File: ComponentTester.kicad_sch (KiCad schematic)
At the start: 15 parts, among them J11 Conn_01x02, J2 Conn_01x03, J3 Conn_01x02, U2 OPA188xxD

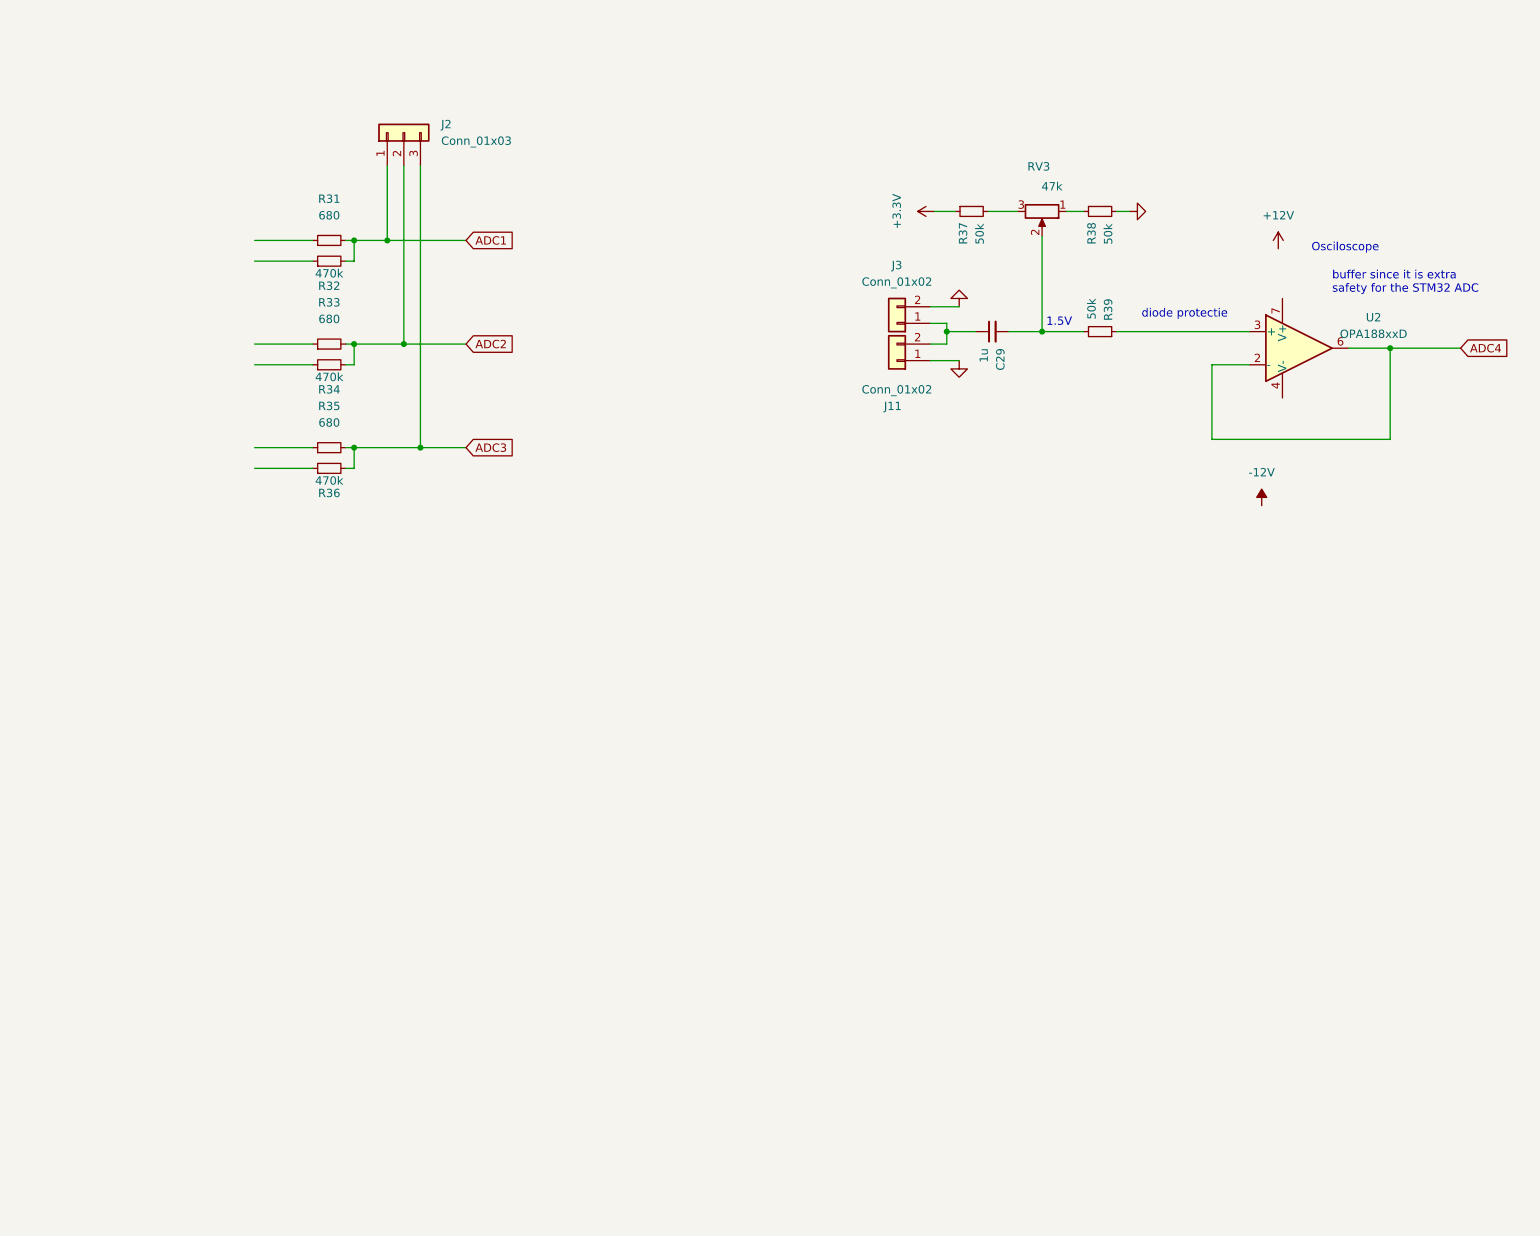
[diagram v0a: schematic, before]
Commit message: more work
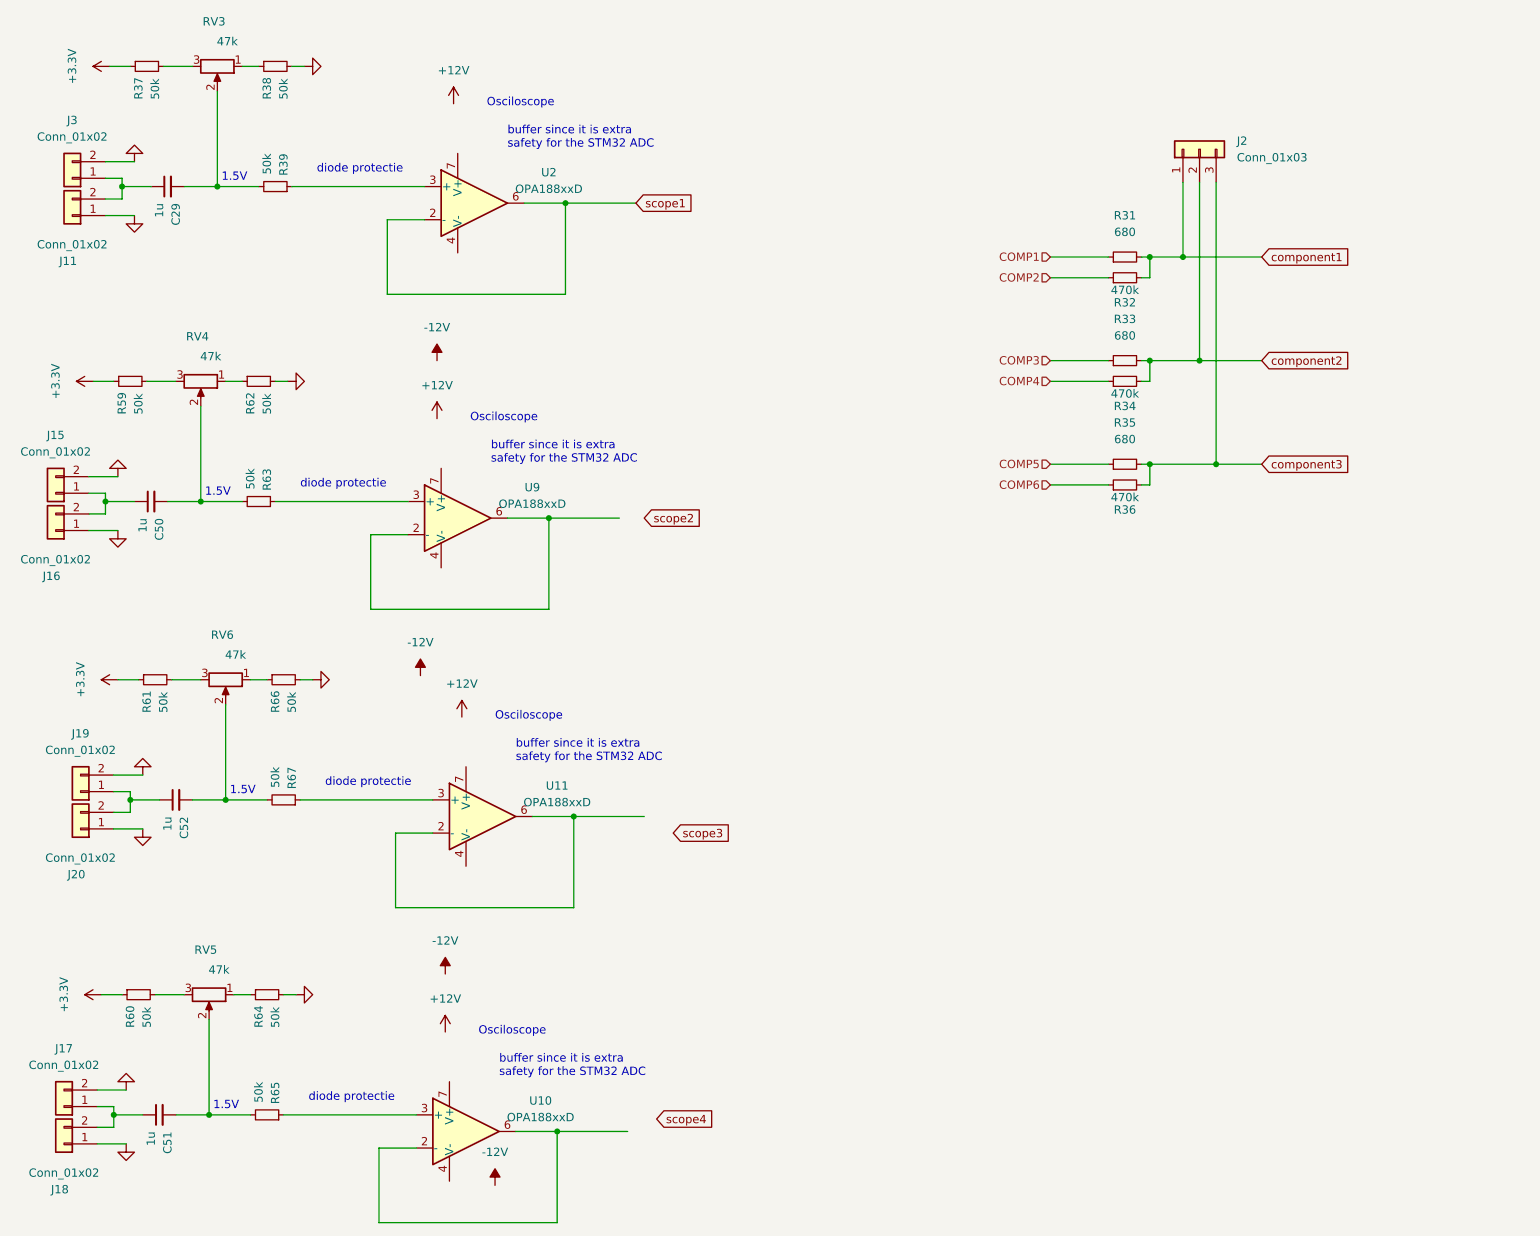
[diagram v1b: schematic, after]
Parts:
- added C50, C51, C52: 1u, Capacitor_SMD:C_0603_1608Metric_Pad1.08x0.95mm_HandSolder, symbol Device:C_Small
- added J15, J16, J17, J18, J19, J20: Conn_01x02, symbol Connector_Generic:Conn_01x02
- added R59, R60, R61, R62, R63, R64, R65, R66, R67: 50k, Resistor_SMD:R_0603_1608Metric_Pad0.98x0.95mm_HandSolder, symbol Device:R_Small
- added RV4, RV5, RV6: 47k, Z_mycustom_footprint_lib:2002102255, symbol Device:R_Potentiometer
- added U10, U11, U9: OPA188xxD, Package_SO:SOIC-8_3.9x4.9mm_P1.27mm, symbol Amplifier_Operational:OPA188xxD
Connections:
- net +3V3: now also R59.1, R60.1, R61.1
- net GND: now also J15.2 (Pin_2), J16.1 (Pin_1), J17.2 (Pin_2), J18.1 (Pin_1), J19.2 (Pin_2), J20.1 (Pin_1), R62.2, R64.2, R66.2
- net COMP5: now reaches R35.1
- net COMP4: now reaches R34.1
- net COMP6: now reaches R36.1
- net COMP1: now reaches R31.1
- net COMP2: now reaches R32.1
- net COMP3: now reaches R33.1
- net ADC1 renamed component1
- net ADC2 renamed component2
- net ADC3 renamed component3
- net ADC4 renamed scope1
- new net: R60.2, RV5.3
- new net: R66.1, RV6.1
- new net: C52.1, J19.1 (Pin_1), J20.2 (Pin_2)
- new net: R67.1, U11.3 (+)
- new net: C52.2, R67.2, RV6.2
- new net: R64.1, RV5.1
- new net: R59.2, RV4.3
- new net: R61.2, RV6.3
- new net: C50.1, J15.1 (Pin_1), J16.2 (Pin_2)
- new net: R65.1, U10.3 (+)
- new net: C51.2, R65.2, RV5.2
- new net: R62.1, RV4.1
- new net: C51.1, J17.1 (Pin_1), J18.2 (Pin_2)
- new net: C50.2, R63.2, RV4.2
- new net: U10.2 (-), U10.6
- new net: U9.2 (-), U9.6
- new net: R63.1, U9.3 (+)
- new net: U11.2 (-), U11.6
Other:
- moved on the sheet: C29, J11, J2, J3, R31, R32, R33, R34, R35, R36, R37, R38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
